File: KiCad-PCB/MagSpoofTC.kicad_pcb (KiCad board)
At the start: 2 copper layers, 35 x 29 mm, 13 parts, among them IC1 ATTINY85-P, P1 Battery, P2 AVR ICSP, SW1 SW_PUSH, U1 TC4424

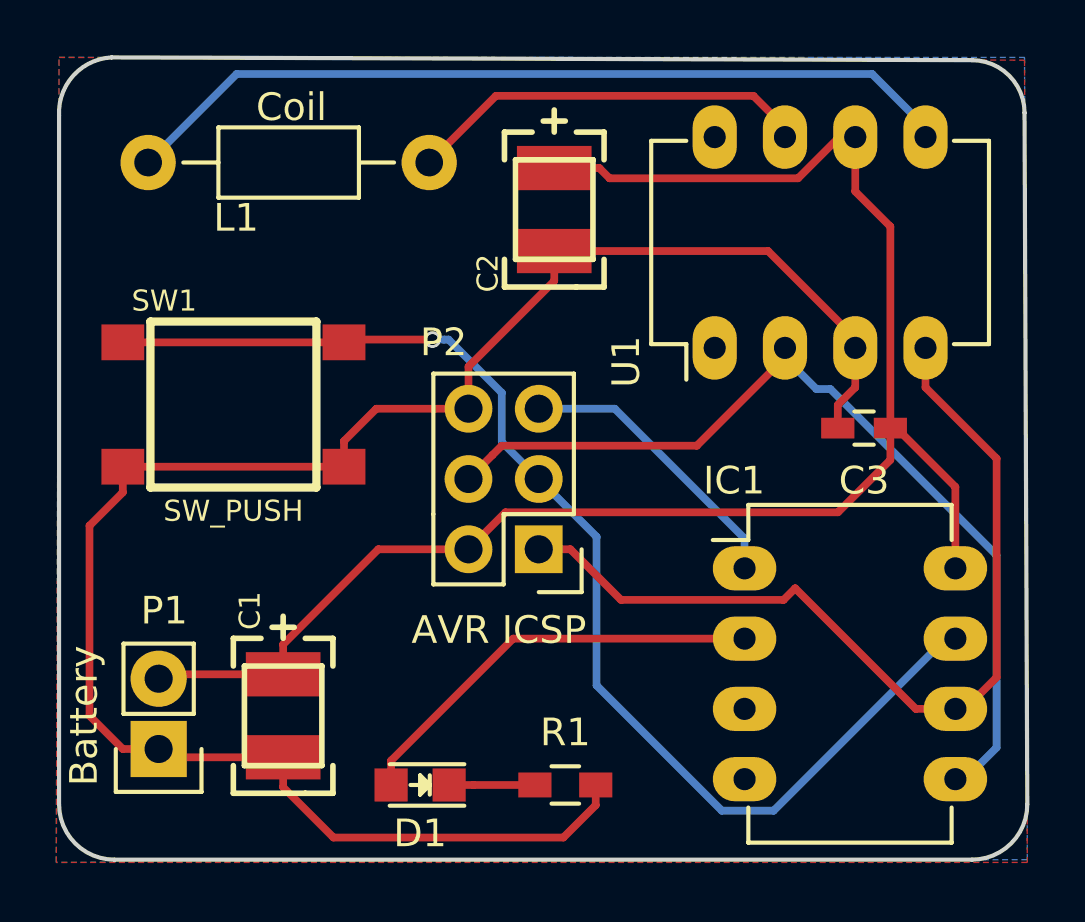
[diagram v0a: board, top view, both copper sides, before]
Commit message: Update version 1.1
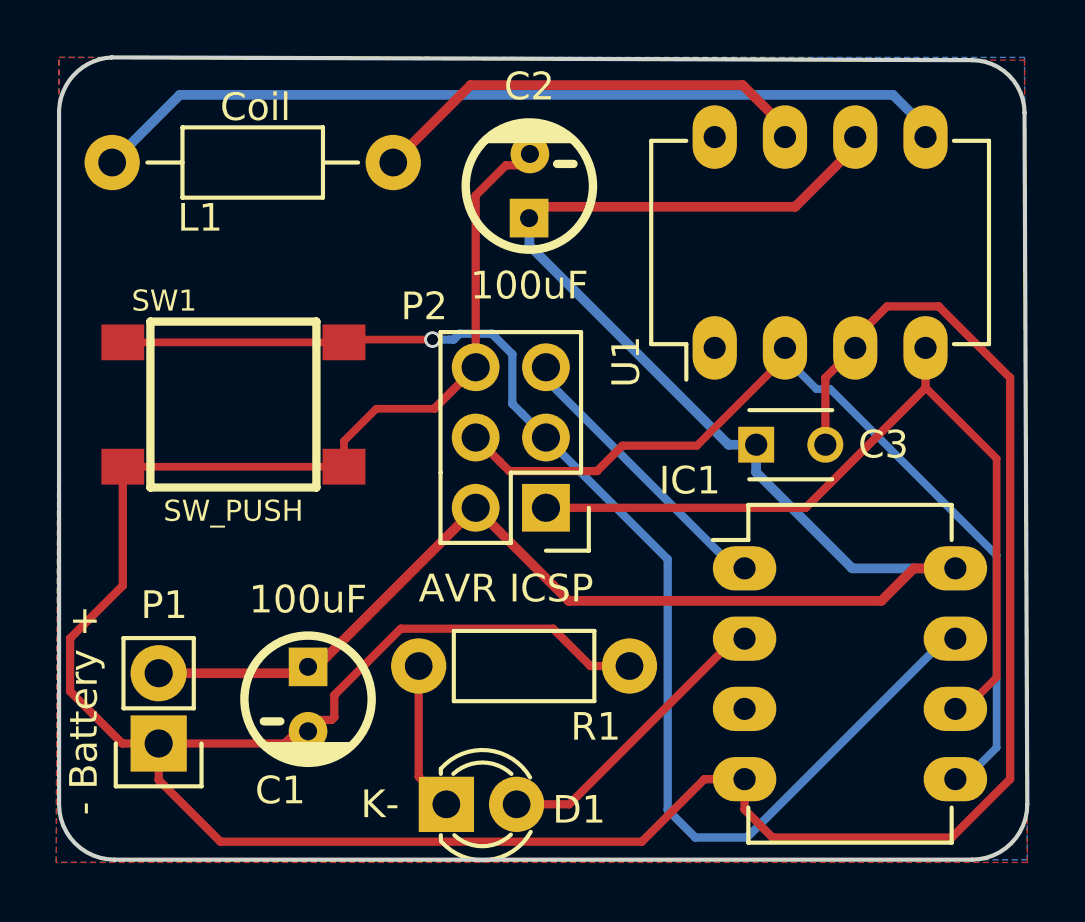
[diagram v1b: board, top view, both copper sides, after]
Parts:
- C1, C2: footprint theinventorhouse:1411(3528m)-B%2CM%2CH%2CT-TANTALUM -> theinventorhouse:CP_4x5mm
- C3: footprint Capacitors_SMD:C_0603_HandSoldering -> Capacitors_ThroughHole:C_Disc_D3_P2.5
- D1: footprint LEDs:LED-0805 -> LEDs:LED-3MM
- P1: value Battery -> - Battery +
- R1: footprint Resistors_SMD:R_0603_HandSoldering -> Resistors_ThroughHole:Resistor_Horizontal_RM7mm
- moved R1 6.82 mm to (116.0, 101.0)
- moved ? 5.10 mm to (109.2, 95.2)
- moved C3 3.95 mm to (128.2, 93.0), turned to 0 degrees
- moved P2 1.52 mm to (120.6, 95.3)
- moved G*** 1.40 mm to (109.8, 88.0)
- moved L1 1.30 mm to (110.0, 82.8)
- moved C2 1.24 mm to (120.0, 83.7), turned to 0 degrees
- moved D1 1.18 mm to (117.0, 106.0), turned to 0 degrees
- moved C1 1.08 mm to (112.0, 102.2), turned to 180 degrees
- moved P1 0.20 mm to (106.6, 103.8)
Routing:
- net GND: track 68.5 -> 119.1 mm
- net VCC: track 61.1 -> 70.1 mm
- net Net-(D1-Pad2): track 15.5 -> 10.7 mm
- net /SCK: track 44.3 -> 47.5 mm
- net Net-(D1-Pad1): track 3.10 -> 5.41 mm
- net Net-(L1-Pad1): track 14.7 -> 16.3 mm
- net /MISO: track 32.7 -> 31.9 mm
- net Net-(L1-Pad2): track 30.6 -> 31.2 mm
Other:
- net class Alimentacion added: clearance 0.2, trace_width 0.35, via_dia 0.6, via_drill 0.4
- net class Default: trace_width 0.28 -> 0.3
- board text added: "MagSpoof 1.1v"
- board text removed: "MagSpoof 1.0v"
